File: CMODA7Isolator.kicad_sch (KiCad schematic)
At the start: 35 parts, among them J1 Conn_01x24, J2 Conn_01x24, M1 Artix_7_35T_CMOD_A7, U1 TXB0108, U2 TXB0108, U3 TXB0108, U4 TXB0108, U5 TXB0108, U6 TXB0108, U7 LD1117S33TR_SOT223

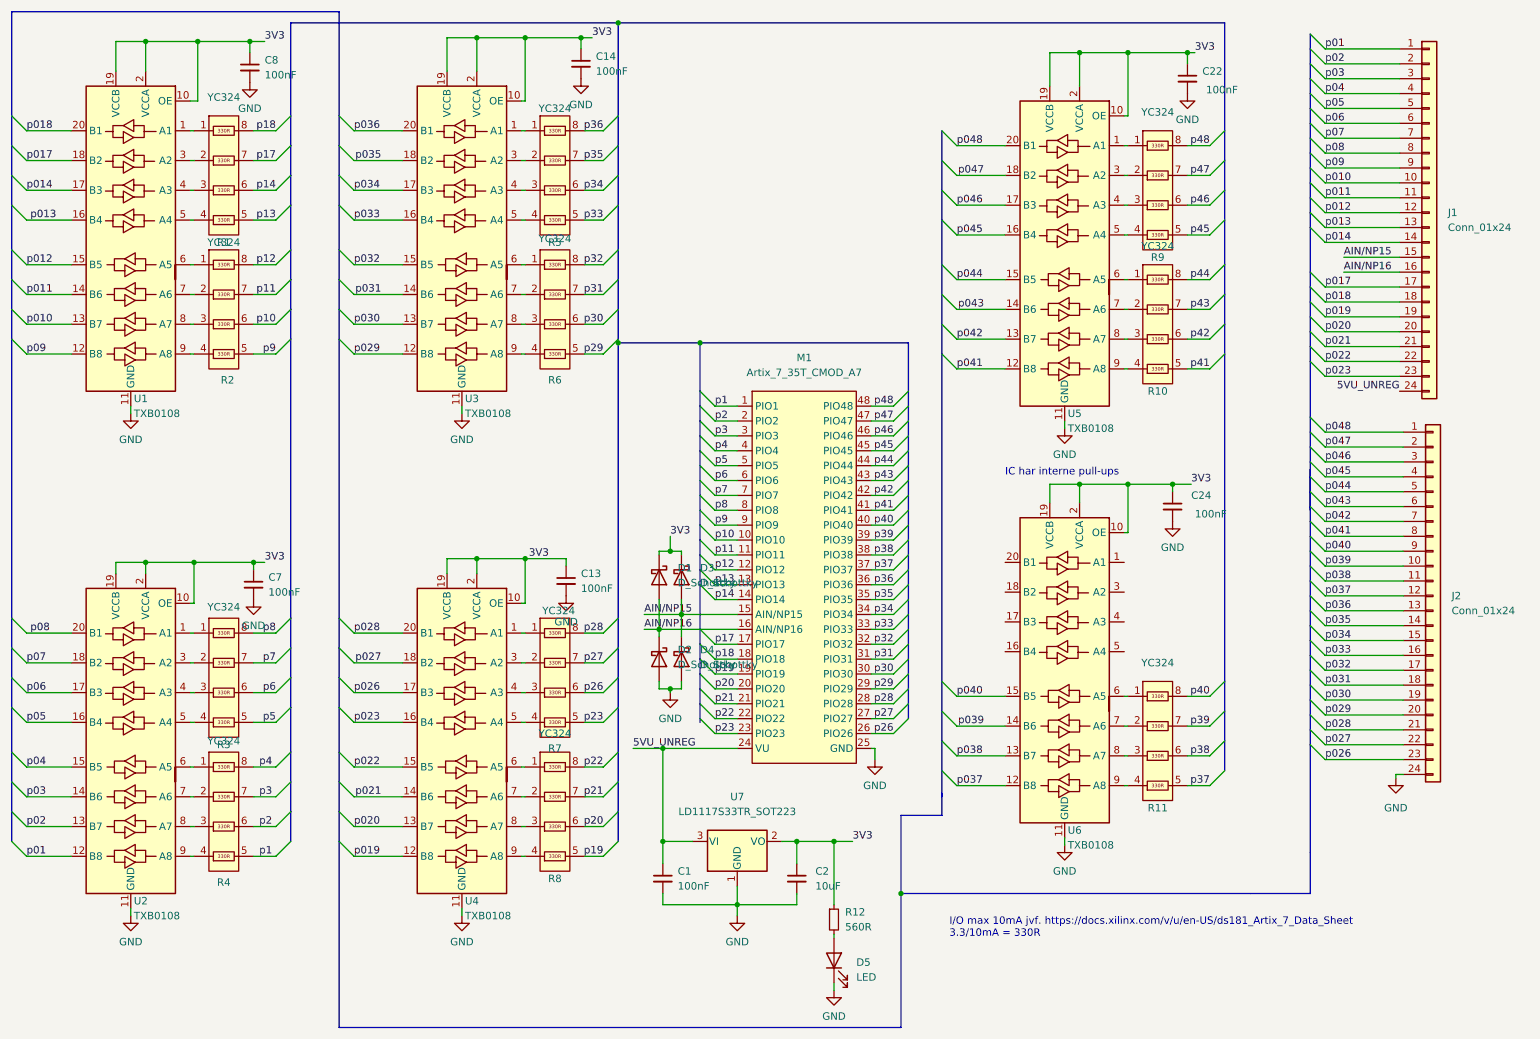
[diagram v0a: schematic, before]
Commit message: Issue #6 fixed
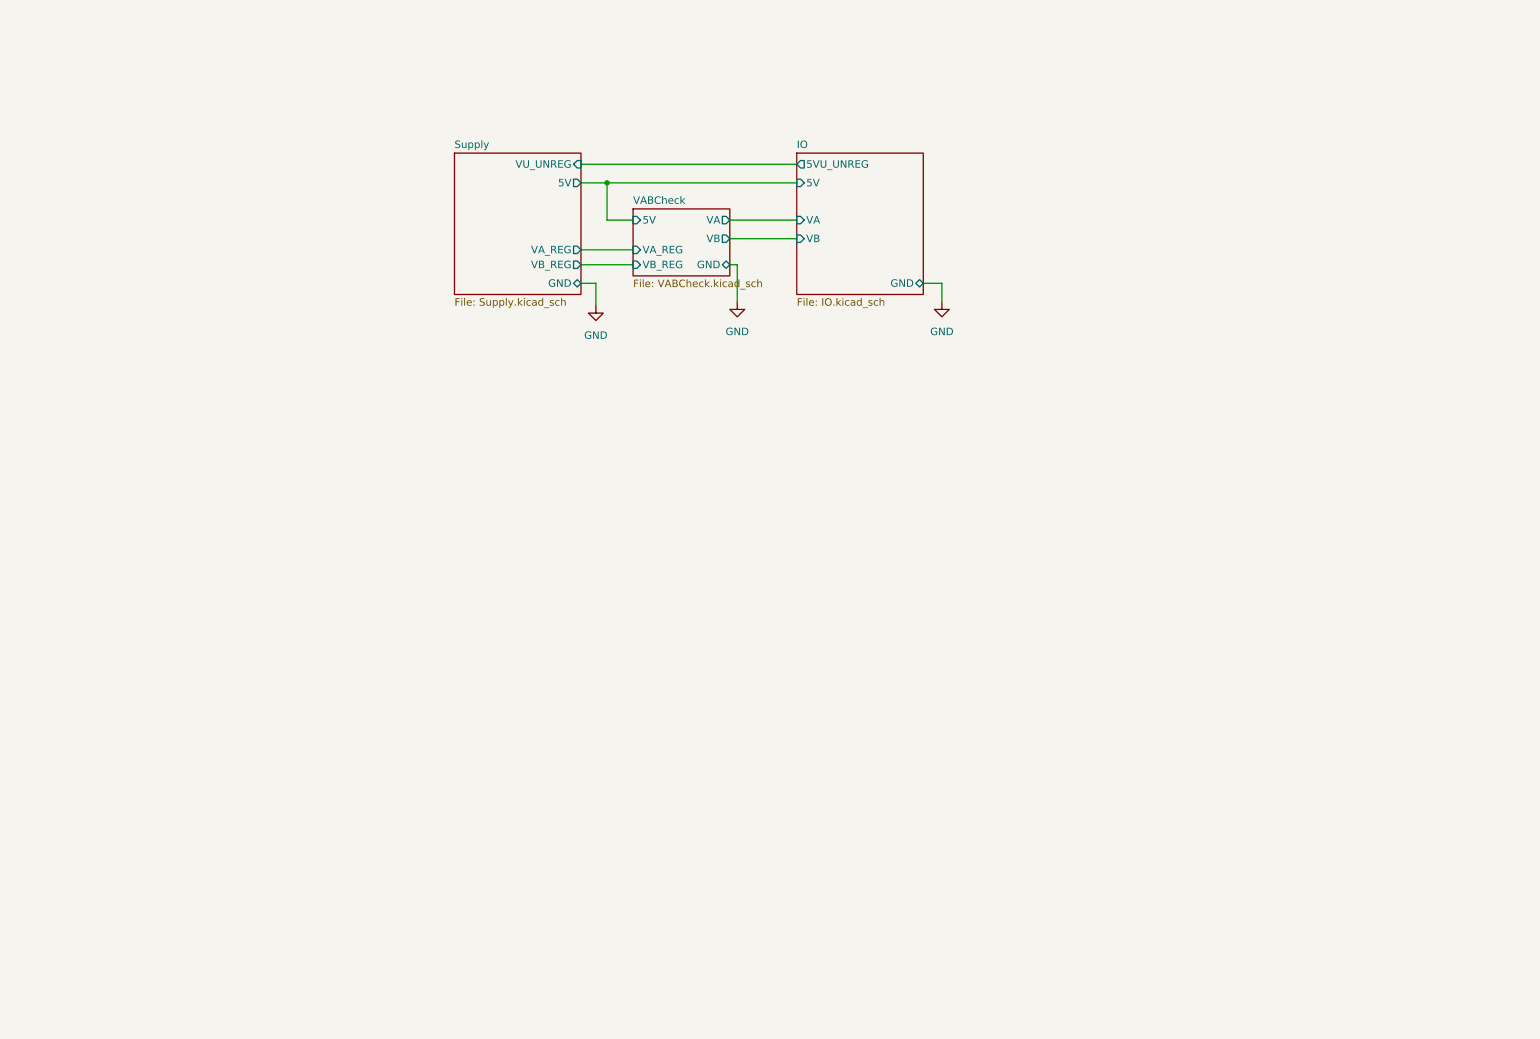
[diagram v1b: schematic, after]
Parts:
- removed C1, C13, C14, C22, C24, C7, C8: 100nF, Capacitor_SMD:C_0805_2012Metric_Pad1.18x1.45mm_HandSolder, symbol Device:C_Small
- removed C2: 10uF, Capacitor_SMD:C_0805_2012Metric_Pad1.18x1.45mm_HandSolder, symbol Device:C_Small
- removed D1, D2, D3, D4: D_Schottky, Diode_SMD:D_SOD-123, symbol Device:D_Schottky
- removed D5: LED, LED_SMD:LED_0603_1608Metric, symbol Device:LED
- removed J1, J2: Conn_01x24, Connector_PinHeader_2.54mm:PinHeader_1x24_P2.54mm_Vertical, symbol Connector_Generic:Conn_01x24
- removed M1: Artix_7_35T_CMOD_A7, JRIX FPGA:CMOD A7 Module, symbol JRIX FPGA:Artix_7_35T_CMOD_A7
- removed R1, R10, R11, R2, R3, R4, R5, R6, R7, R8, R9: YC324, JRIX Resistor Array Footprints:YC-TC 124 8Pin-4R, symbol JRIX Resistor Array:YC324
- removed R12: 560R, Resistor_SMD:R_0805_2012Metric_Pad1.20x1.40mm_HandSolder, symbol Device:R_Small
- removed U1, U2, U3, U4, U5, U6: TXB0108, Package_SO:TSSOP-20_4.4x6.5mm_P0.65mm, symbol JRIX Level Translator:TXB0108
- removed U7: LD1117S33TR_SOT223, Package_TO_SOT_SMD:SOT-223-3_TabPin2, symbol Regulator_Linear:LD1117S33TR_SOT223
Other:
- added sheet IO (IO.kicad_sch)
- added sheet Supply (Supply.kicad_sch)
- added sheet VABCheck (VABCheck.kicad_sch)
- note removed: "I/O max 10mA jvf. https://docs.xilinx.com/v/u/en-US/ds181_Artix_7_Data_Sheet 3.3/10mA = 330R"
- note removed: "IC har interne pull-ups"
